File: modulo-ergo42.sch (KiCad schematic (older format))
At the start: 4 parts

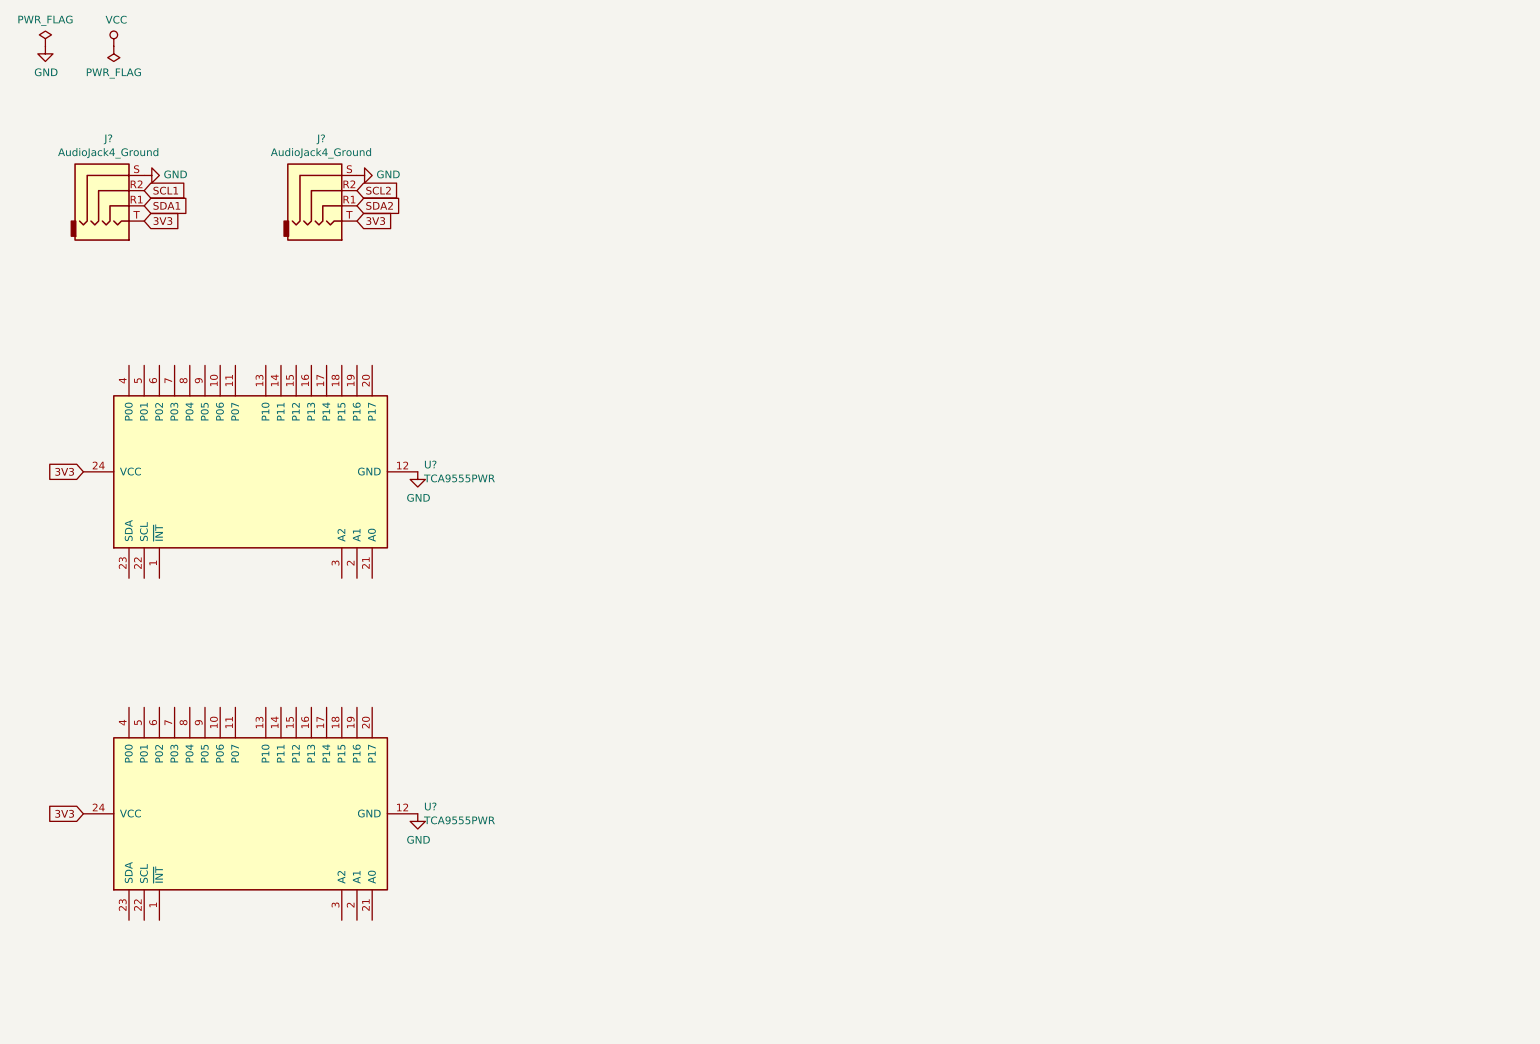
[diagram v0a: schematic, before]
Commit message: Design schematic
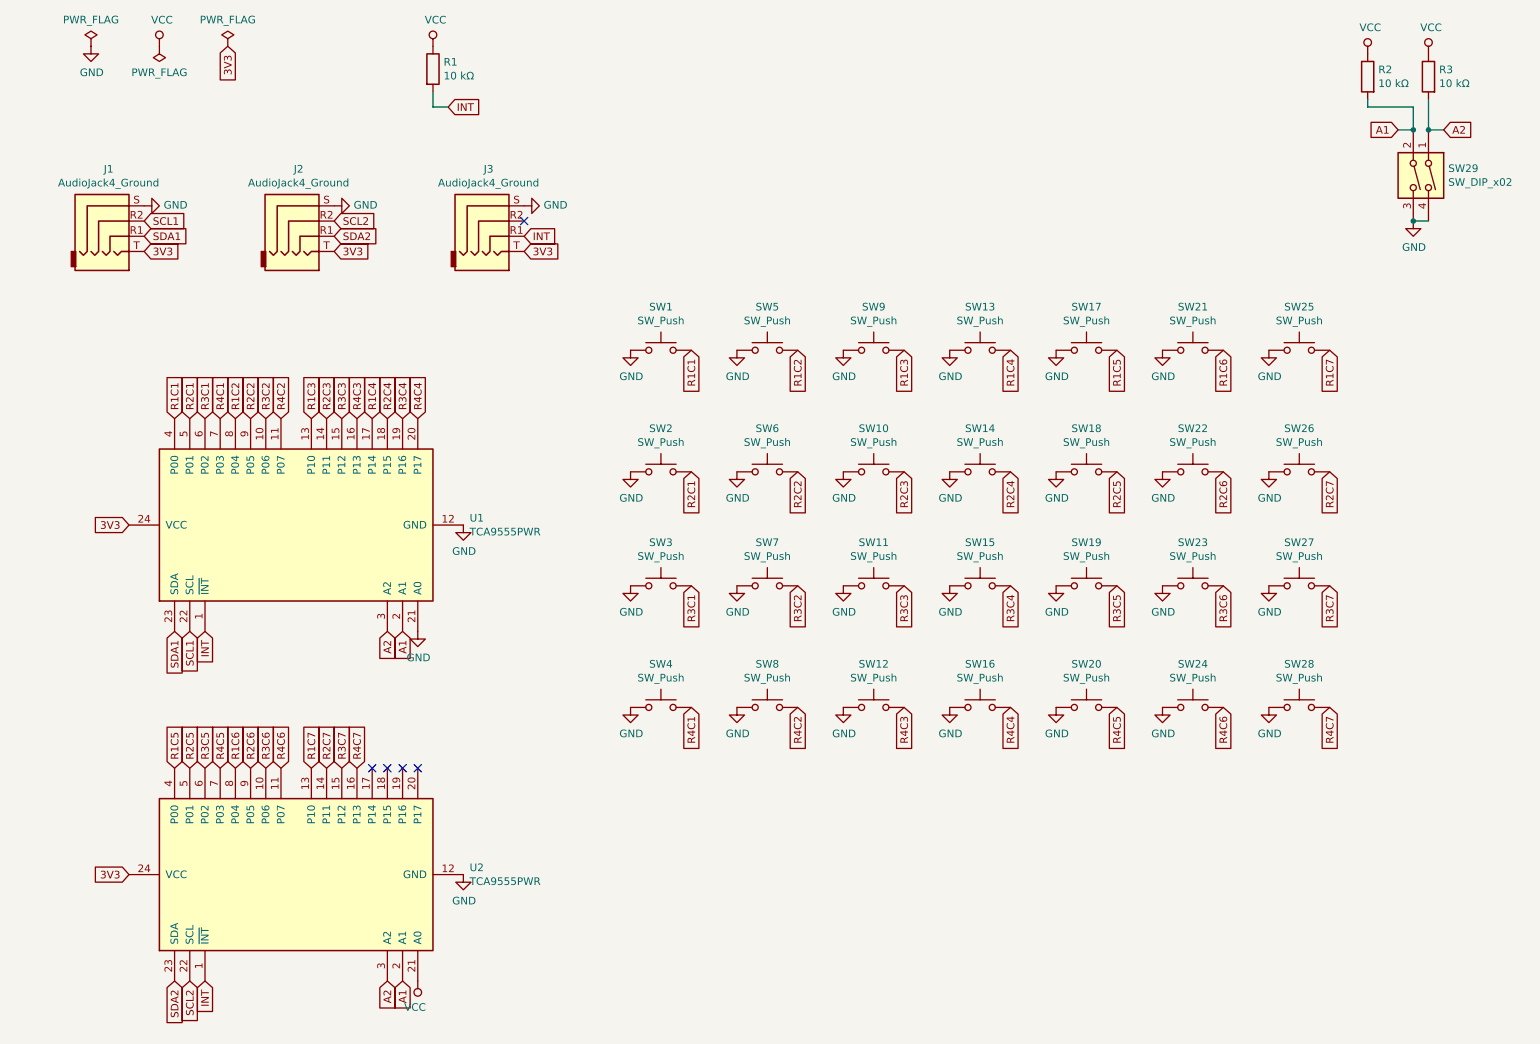
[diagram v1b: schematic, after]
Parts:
- added J3: AudioJack4_Ground, library:TRRS_SMD_PJ320, symbol Connector:AudioJack4_Ground
- added R1, R2, R3: 10 kΩ, Resistor_SMD:R_0603_1608Metric, symbol Device:R
- added SW1, SW10, SW11, SW12, SW13, SW14, SW15, SW16, SW17, SW18, SW19, SW2, SW20, SW21, SW22, SW23, SW24, SW25, SW26, SW27, SW28, SW3, SW4, SW5, SW6, SW7, SW8, SW9: SW_Push, library:Kailh_Socket, symbol Switch:SW_Push
- added SW29: SW_DIP_x02, library:DipSwitch, symbol Switch:SW_DIP_x02
- J1, J2: renamed from J?; footprint (none) -> library:TRRS_SMD_PJ320
- gave numbers to parts that had none: 2
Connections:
- net 3V3: now also J3.T
- net GND: now also U1.21 (A0), J3.S, SW1.1, SW10.1, SW11.1, SW12.1, SW13.1, SW14.1, SW15.1, SW16.1, SW17.1, SW18.1, SW19.1, SW2.1, SW20.1, SW21.1, SW22.1, SW23.1, SW24.1, SW25.1, SW26.1, SW27.1, SW28.1, SW29.3, SW29.4, SW3.1, SW4.1, SW5.1, SW6.1, SW7.1, SW8.1, SW9.1
- net SCL1: now also U1.22 (SCL)
- net SCL2: now also U2.22 (SCL)
- net SDA1: now also U1.23 (SDA)
- net SDA2: now also U2.23 (SDA)
- net VCC: now also U2.21 (A0), R1.1, R2.1, R3.1
- net INT: now reaches U1.1 (~INT)
- net INT: now also U2.1 (~INT), J3.R1, R1.2
- net R3C2: now reaches U1.10 (P06)
- net R3C2: now also SW7.2
- net R4C2: now reaches U1.11 (P07)
- net R4C2: now also SW8.2
- net R1C3: now reaches U1.13 (P10)
- net R1C3: now also SW9.2
- net R2C3: now reaches U1.14 (P11)
- net R2C3: now also SW10.2
- net R3C3: now reaches U1.15 (P12)
- net R3C3: now also SW11.2
- net R4C3: now reaches U1.16 (P13)
- net R4C3: now also SW12.2
- net R1C4: now reaches U1.17 (P14)
- net R1C4: now also SW13.2
- net R2C4: now reaches U1.18 (P15)
- net R2C4: now also SW14.2
- net R3C4: now reaches U1.19 (P16)
- net R3C4: now also SW15.2
- net A1: now reaches U1.2 (A1)
- net A1: now also U2.2 (A1), R2.2, SW29.2
- net R4C4: now reaches U1.20 (P17)
- net R4C4: now also SW16.2
- net A2: now reaches U1.3 (A2)
- net A2: now also U2.3 (A2), R3.2, SW29.1
- net R1C1: now reaches U1.4 (P00)
- net R1C1: now also SW1.2
- net R2C1: now reaches U1.5 (P01)
- net R2C1: now also SW2.2
- net R3C1: now reaches U1.6 (P02)
- net R3C1: now also SW3.2
- net R4C1: now reaches U1.7 (P03)
- net R4C1: now also SW4.2
- net R1C2: now reaches U1.8 (P04)
- net R1C2: now also SW5.2
- net R2C2: now reaches U1.9 (P05)
- net R2C2: now also SW6.2
- net R3C6: now reaches U2.10 (P06)
- net R3C6: now also SW23.2
- net R4C6: now reaches U2.11 (P07)
- net R4C6: now also SW24.2
- net R1C7: now reaches U2.13 (P10)
- net R1C7: now also SW25.2
- net R2C7: now reaches U2.14 (P11)
- net R2C7: now also SW26.2
- net R3C7: now reaches U2.15 (P12)
- net R3C7: now also SW27.2
- net R4C7: now reaches U2.16 (P13)
- net R4C7: now also SW28.2
- net R1C5: now reaches U2.4 (P00)
- net R1C5: now also SW17.2
- net R2C5: now reaches U2.5 (P01)
- net R2C5: now also SW18.2
- net R3C5: now reaches U2.6 (P02)
- net R3C5: now also SW19.2
- net R4C5: now reaches U2.7 (P03)
- net R4C5: now also SW20.2
- net R1C6: now reaches U2.8 (P04)
- net R1C6: now also SW21.2
- net R2C6: now reaches U2.9 (P05)
- net R2C6: now also SW22.2
- no-connect marks 0 -> 5
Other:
- moved on the sheet: J1, J2, U1, U2
